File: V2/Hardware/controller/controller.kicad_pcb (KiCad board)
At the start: 2 copper layers, 50 parts, among them J0 Molex_PSU_F, J2 Flat_7seg_F, J3 Rpi_DATA_F_3.3V, Q0 BD139-16, Q1 BD139-16, Q2 BD139-16, Q3 BD139-16, Q4 BD139-16, Q5 BD139-16, Q6 BD139-16, U1 ATtiny2313-20PU

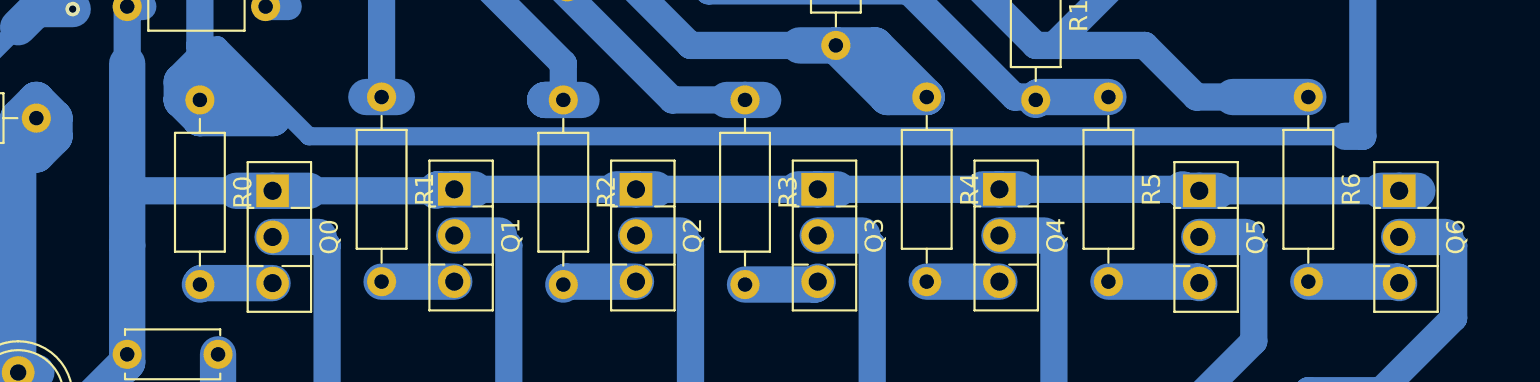
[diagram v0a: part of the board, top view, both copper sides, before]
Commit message: Add kicad part lists
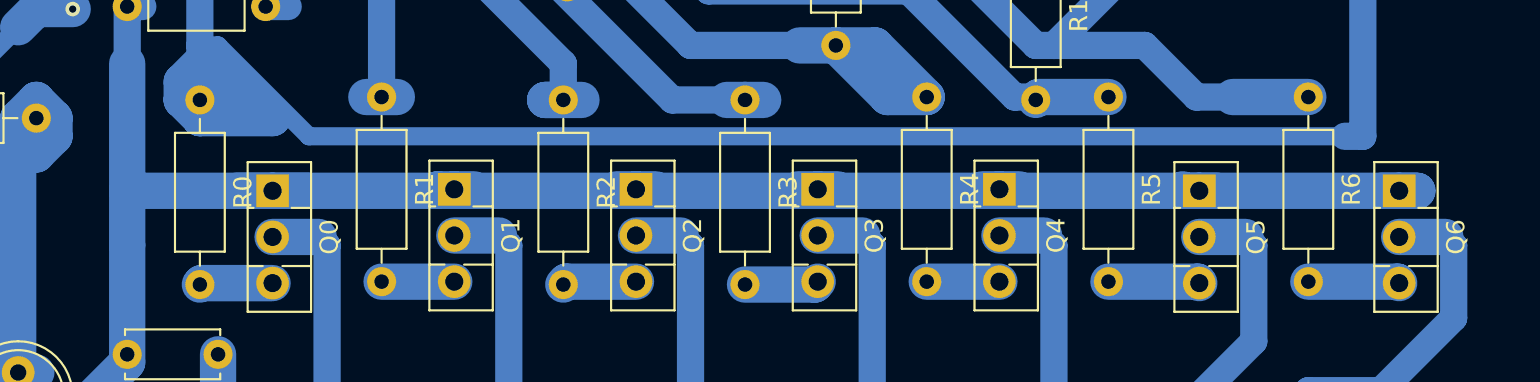
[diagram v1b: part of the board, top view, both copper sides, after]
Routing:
- net Earth: track 443.3 -> 514.3 mm
